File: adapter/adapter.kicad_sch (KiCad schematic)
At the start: 20 parts, among them J1 Serial, J10 Ribbon, J2 Serial, J3 RGB, J4 RGB, J5 Trackball, J6 Ribbon, J7 Trackball, J8 Ribbon, J9 Ribbon, U1 STM32F401 / STM32F411 Blackpi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, U2 STM32F401 / STM32F411 Blackpi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

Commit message: right edge cuts
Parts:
- J9: footprint customs:PinHeader_1x05_P2.54mm_Vertical -> Connector_PinHeader_2.54mm:PinHeader_1x05_P2.54mm_Vertical
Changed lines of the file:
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@@
       (effects (font (size 1.27 1.27)) (justify left))
     )
-    (property "Footprint" "customs:PinHeader_1x05_P2.54mm_Vertical" (id 2) (at 233.299 67.691 0)
+    (property "Footprint" "Connector_PinHeader_2.54mm:PinHeader_1x05_P2.54mm_Vertical" (id 2) (at 233.299 67.691 0)
       (effects (font (size 1.27 1.27)) hide)
     )
@@
     )
     (path "/fcc4bfec-a658-4f05-a805-e2fbe77edcaf"
-      (reference "J9") (unit 1) (value "Ribbon") (footprint "customs:PinHeader_1x05_P2.54mm_Vertical")
+      (reference "J9") (unit 1) (value "Ribbon") (footprint "Connector_PinHeader_2.54mm:PinHeader_1x05_P2.54mm_Vertical")
     )
     (path "/72f9f857-8d29-4f7f-9028-4223dc06e9cc"

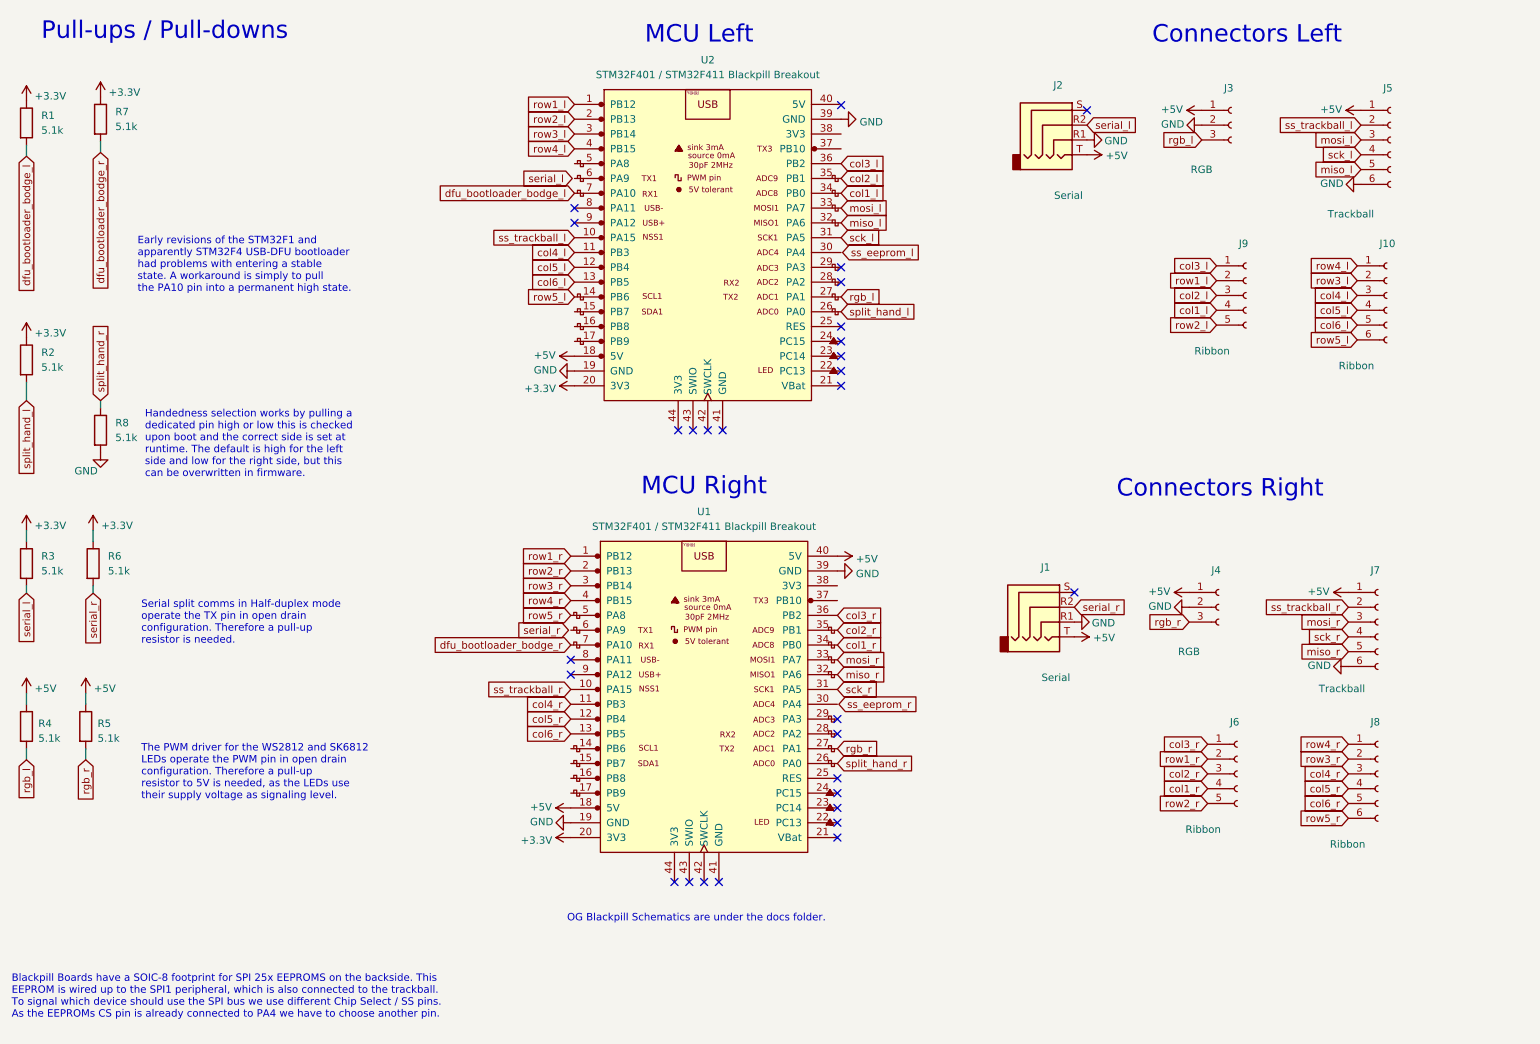
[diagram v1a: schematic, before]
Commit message: Traces for left side
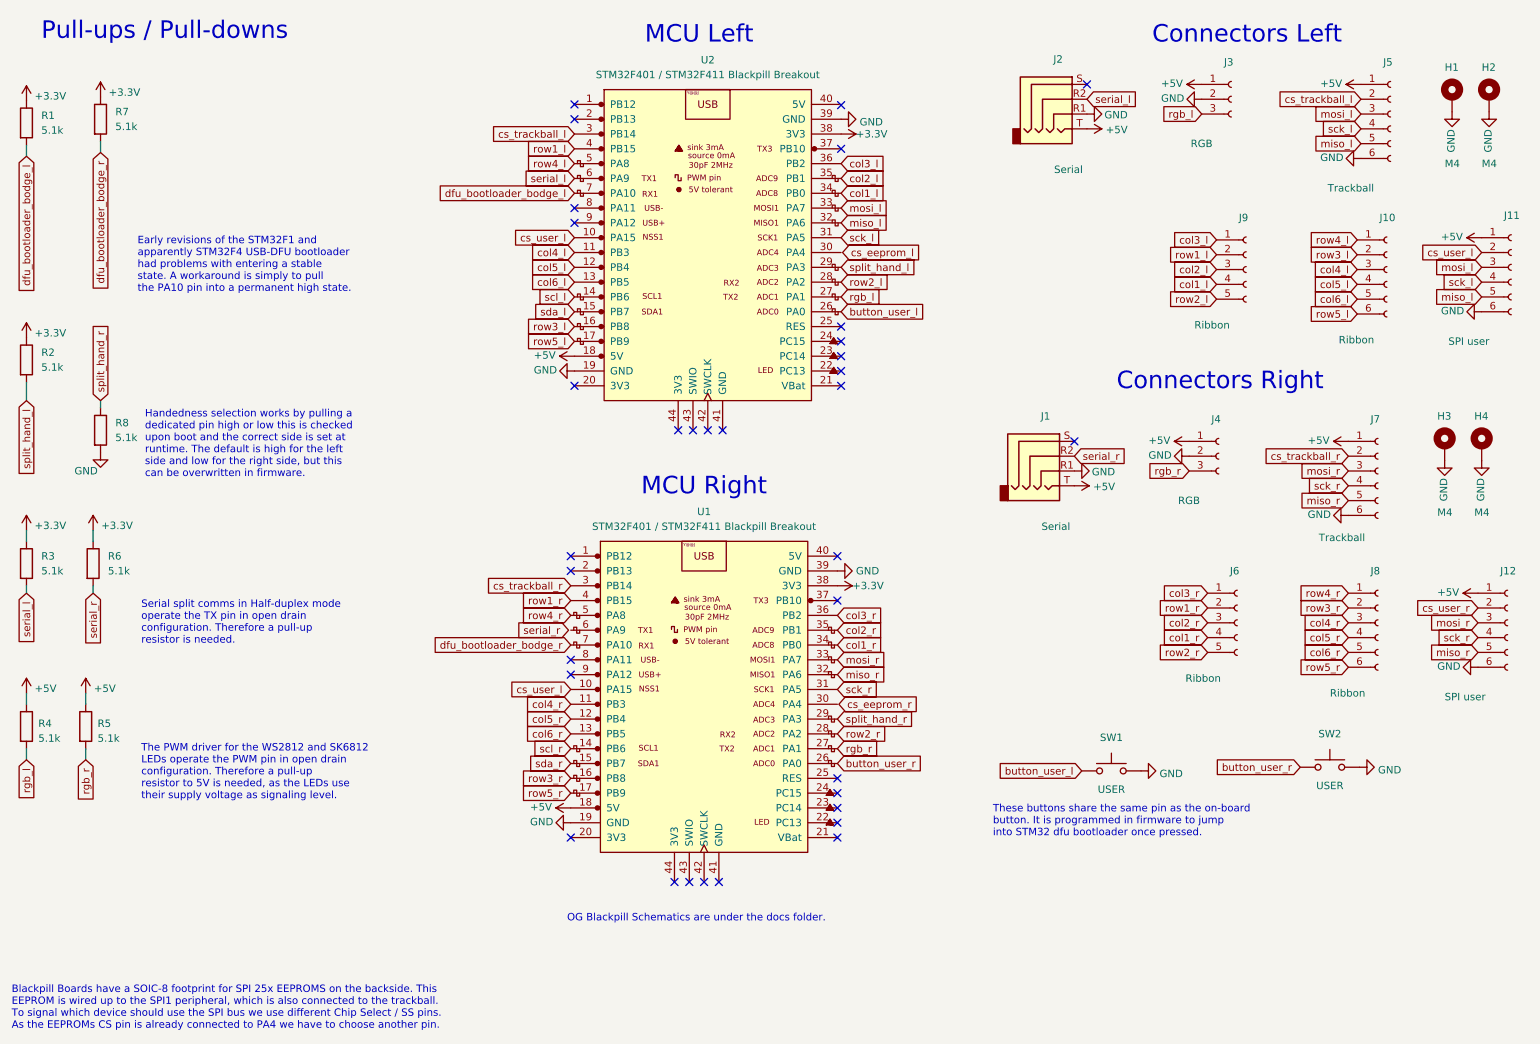
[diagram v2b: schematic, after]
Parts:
- added H1, H2, H3, H4: M4, Library:MountingHole_4mm_Pad_Thin, symbol Mechanical:MountingHole_Pad
- added J11, J12: SPI user, Library:6_PinHeader, symbol Connector:Conn_01x06_Female
- added SW1, SW2: USER, Library:PushSwitch, symbol Switch:SW_Push
- J10, J5, J7, J8: footprint Connector_PinHeader_2.54mm:PinHeader_1x06_P2.54mm_Vertical -> Library:6_PinHeader
- J3, J4: footprint Connector_PinSocket_2.54mm:PinSocket_1x03_P2.54mm_Vertical -> Library:3_PinSocket
- J6, J9: footprint Connector_PinHeader_2.54mm:PinHeader_1x05_P2.54mm_Vertical -> Library:5_PinHeader
- R1, R2, R3, R4, R5, R6, R7, R8: JLCPCB Part C27834 -> C26033
- U1, U2: footprint Library:YAAJ_WeAct_BlackPill_SWD_2 -> Library:WeAct_BlackPill_without_SWD_First_Row
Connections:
- net +3V3: now also U1.38 (3V3), U2.38 (3V3); no longer U1.20 (3V3), U2.20 (3V3)
- net +5V: now also J11.1 (Pin_1), J12.1 (Pin_1); no longer U1.40 (5V)
- net GND: now also H1.1, H2.1, H3.1, H4.1, J11.6 (Pin_6), J12.6 (Pin_6), SW1.2, SW2.2
- net miso_l: now also J11.5 (Pin_5)
- net miso_r: now also J12.5 (Pin_5)
- net mosi_l: now also J11.3 (Pin_3)
- net mosi_r: now also J12.3 (Pin_3)
- net row1_l: now also U2.4 (PB15); no longer U2.1 (PB12)
- net row1_r: now also U1.4 (PB15); no longer U1.1 (PB12)
- net row2_l: now also U2.28 (PA2); no longer U2.2 (PB13)
- net row2_r: now also U1.28 (PA2); no longer U1.2 (PB13)
- net row3_l: now also U2.16 (PB8); no longer U2.3 (PB14)
- net row3_r: now also U1.16 (PB8); no longer U1.3 (PB14)
- net row4_l: now also U2.5 (PA8); no longer U2.4 (PB15)
- net row4_r: now also U1.5 (PA8); no longer U1.4 (PB15)
- net row5_l: now also U2.17 (PB9); no longer U2.14 (PB6)
- net row5_r: now also U1.17 (PB9); no longer U1.5 (PA8)
- net sck_l: now also J11.4 (Pin_4)
- net sck_r: now also J12.4 (Pin_4)
- net serial_l: now also U2.6 (PA9)
- net split_hand_l: now also U2.29 (PA3); no longer U2.26 (PA0)
- net split_hand_r: now also U1.29 (PA3); no longer U1.26 (PA0)
- net scl_r: now reaches U1.14 (PB6)
- net sda_r: now reaches U1.15 (PB7)
- net sda_l: now reaches U2.15 (PB7)
- net ss_trackball_l renamed cs_trackball_l
- net cs_trackball_l: now also U2.3 (PB14); no longer U2.10 (PA15)
- net ss_trackball_r renamed cs_trackball_r
- net cs_trackball_r: now also U1.3 (PB14); no longer U1.10 (PA15)
- new net button_user_l: SW1.1, U2.26 (PA0)
- new net button_user_r: SW2.1, U1.26 (PA0)
- new net cs_user_l: J11.2 (Pin_2), U1.10 (PA15), U2.10 (PA15)
- new net cs_user_r: J12.2 (Pin_2)
- new net scl_l: U2.14 (PB6)
- no-connect marks 29 -> 34
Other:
- note added: "These buttons share the same pin as the on-board button. It is programmed in firmware to jump into STM32 dfu bootloader once pressed."
- moved on the sheet: J1, J10, J2, J3, J4, J5, J6, J7, J8, J9
